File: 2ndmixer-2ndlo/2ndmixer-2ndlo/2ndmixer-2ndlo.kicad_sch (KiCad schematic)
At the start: 58 parts, among them J201 Coax Solder Point, J202 Conn_01x02, J203 Coax Solder Point, Q201 2N5179, Q202 2N5179, T201 Bifilar_Transformer, U201 MAV-11, U202 TUF-1H+, Y201 100MHz

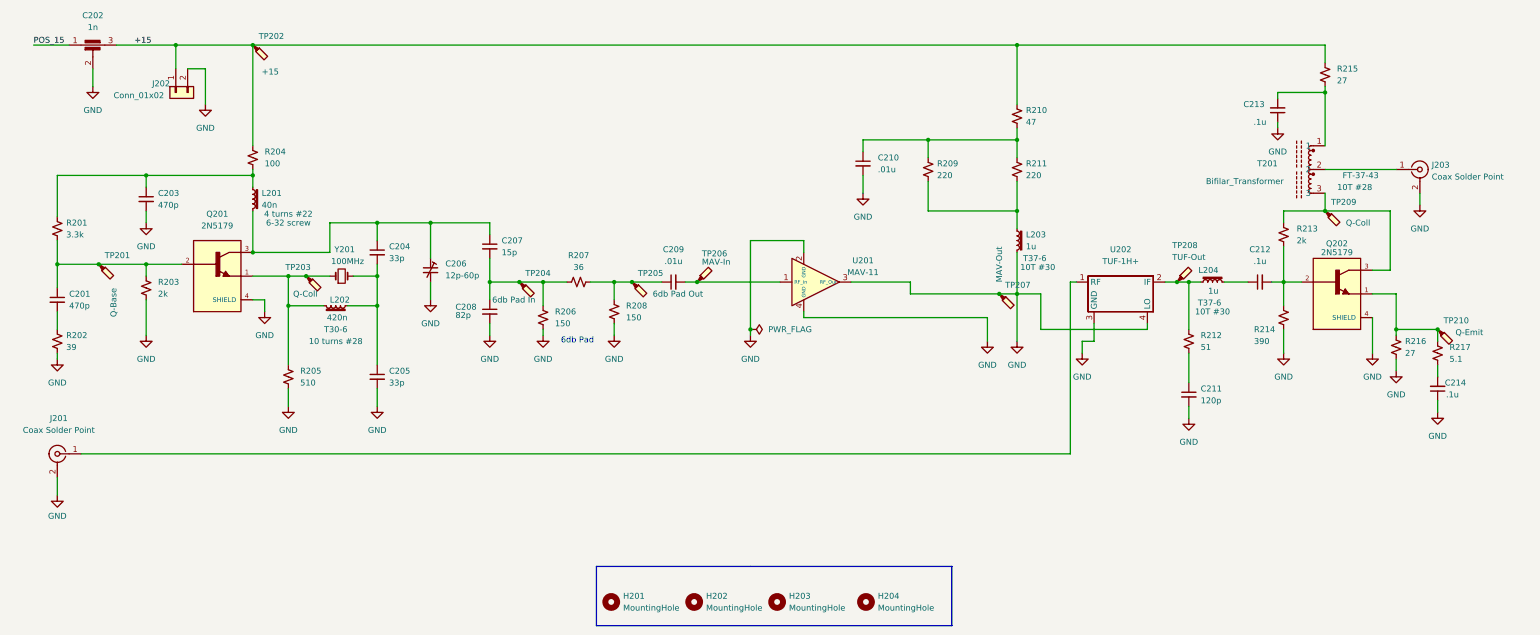
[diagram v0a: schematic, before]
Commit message: v7 conversion
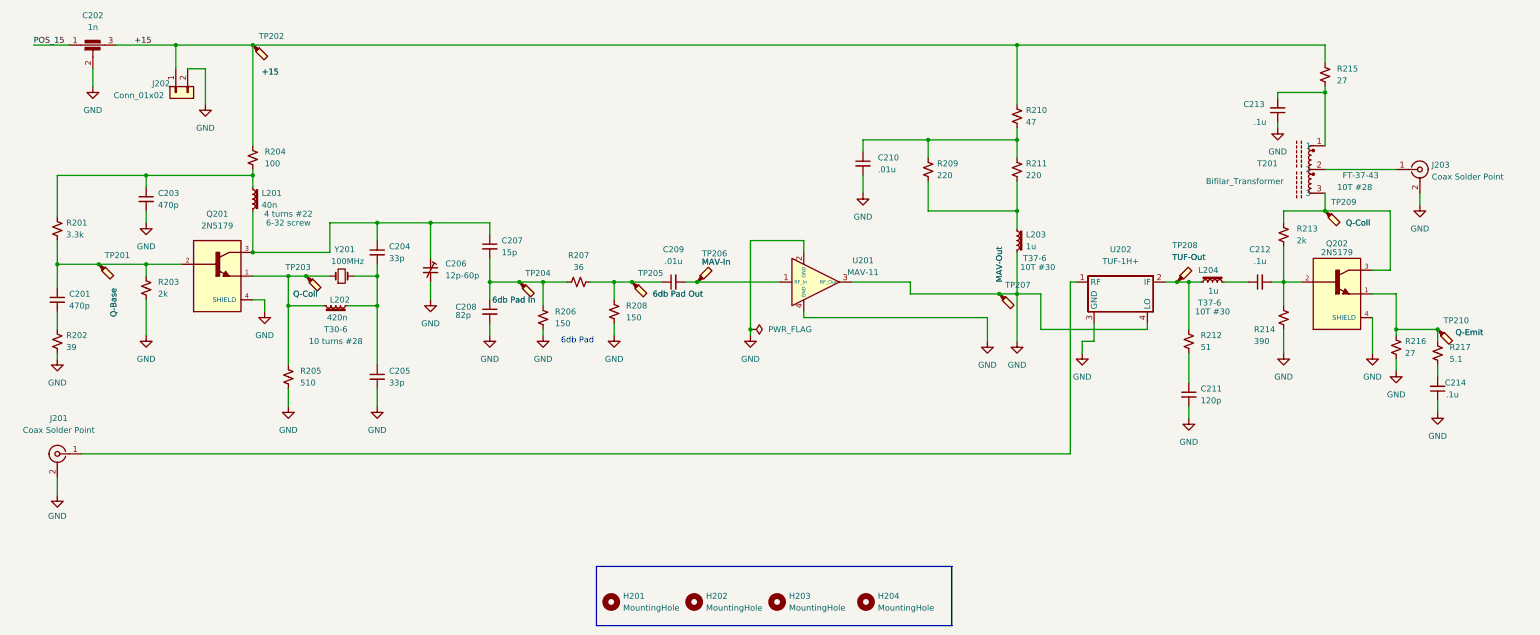
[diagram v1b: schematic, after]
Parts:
- J201, J203: Spice_Model Conn_Coaxial -> (none); Spice_Netlist_Enabled N -> (none); Spice_Primitive J -> (none)
- J202: Spice_Model Conn_01x02 -> (none); Spice_Netlist_Enabled N -> (none); Spice_Primitive J -> (none)
- Q201, Q202: Spice_Lib_File 2ndmixer-2ndlo-spice\2N5179.LIB -> (none); Spice_Model 2N5179 -> (none); Spice_Netlist_Enabled Y -> (none); Spice_Primitive Q -> (none)
- TP201: value Q-Base -> ${SIM.PARAMS}; Spice_Netlist_Enabled N -> (none)
- TP202: value +15 -> ${SIM.PARAMS}; Spice_Netlist_Enabled N -> (none)
- TP203, TP209: value Q-Coll -> ${SIM.PARAMS}; Spice_Netlist_Enabled N -> (none)
- TP204: value 6db Pad In -> ${SIM.PARAMS}; Spice_Netlist_Enabled N -> (none)
- TP205: value 6db Pad Out -> ${SIM.PARAMS}; Spice_Netlist_Enabled N -> (none)
- TP206: value MAV-In -> ${SIM.PARAMS}; Spice_Netlist_Enabled N -> (none)
- TP207: value MAV-Out -> ${SIM.PARAMS}; Spice_Netlist_Enabled N -> (none)
- TP208: value TUF-Out -> ${SIM.PARAMS}; Spice_Netlist_Enabled N -> (none)
- TP210: value Q-Emit -> ${SIM.PARAMS}; Spice_Netlist_Enabled N -> (none)
